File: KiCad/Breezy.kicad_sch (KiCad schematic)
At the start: 23 parts, among them J1 AC Input 120VAC / 5 A / 600W 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, J2 AC Output 120VAC / 5 A / 600W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, J3 AC Input 120VAC / 5 A / 600W 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, J4 AC Output 120VAC / 5 A / 600W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, K1 5V, Q1 2N3904, SW1 Manual Enable, SW2 Automatic Mode Select

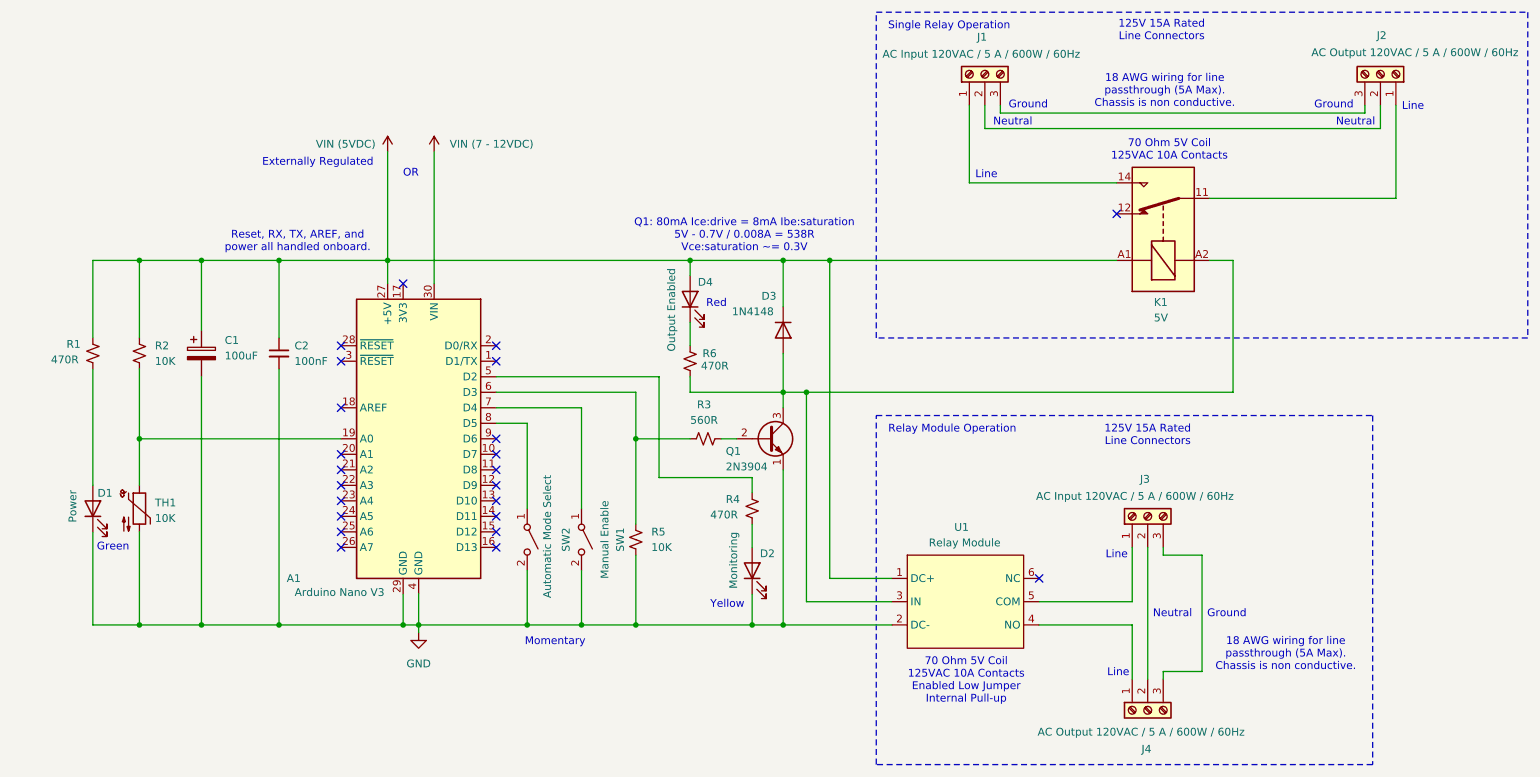
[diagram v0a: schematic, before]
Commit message: Updates
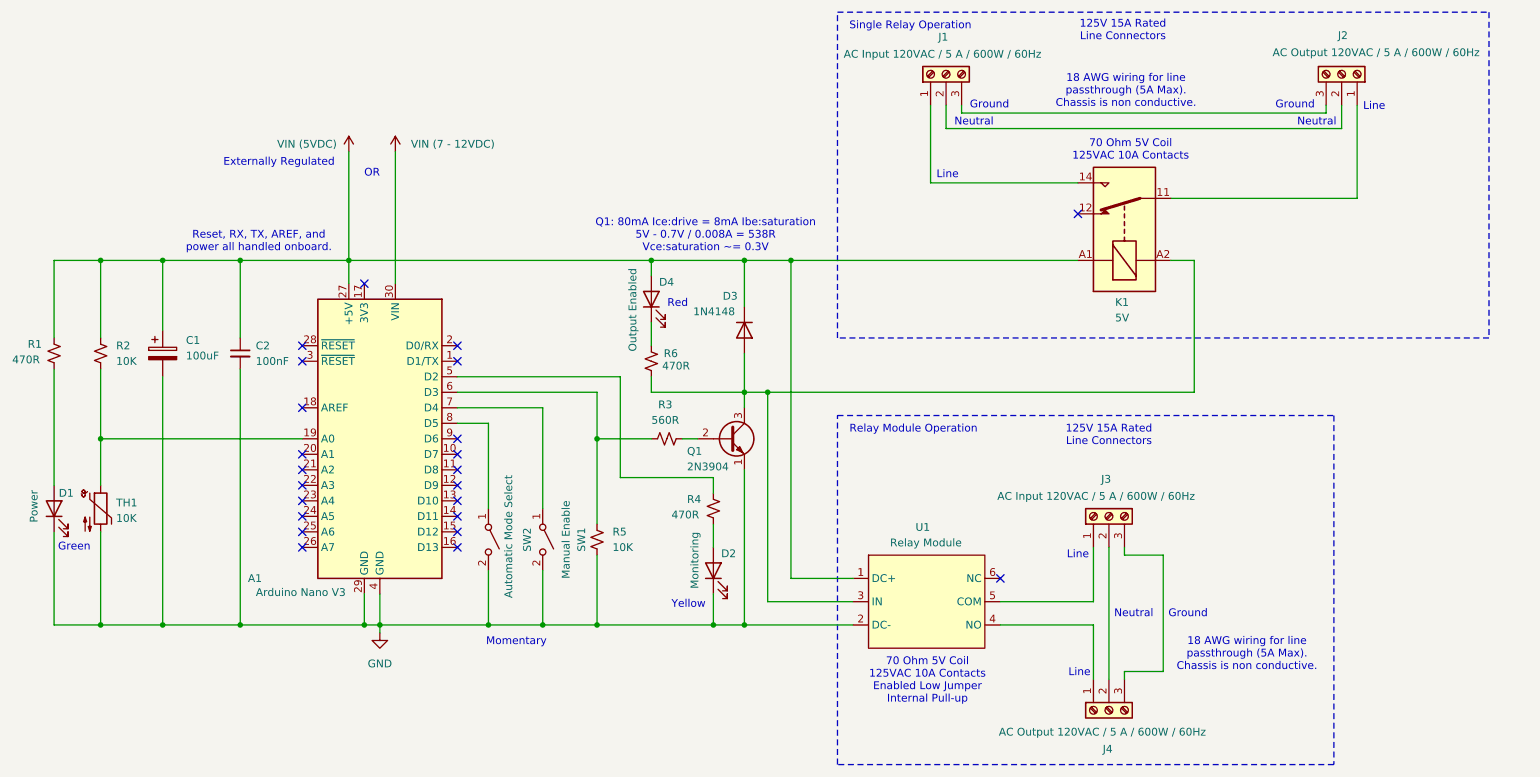
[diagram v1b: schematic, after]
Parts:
- U1: value ~ -> (none)
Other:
- moved on the sheet: A1, C1, C2, D1, D2, D3, D4, J1, J2, J3, J4, K1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
